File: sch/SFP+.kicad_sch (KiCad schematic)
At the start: 13 parts, among them J14 Conn_01x02_Pin, J15 Conn_01x02_Pin, J16 TE 2007262-1, J6 SFP+, J7 SFP+

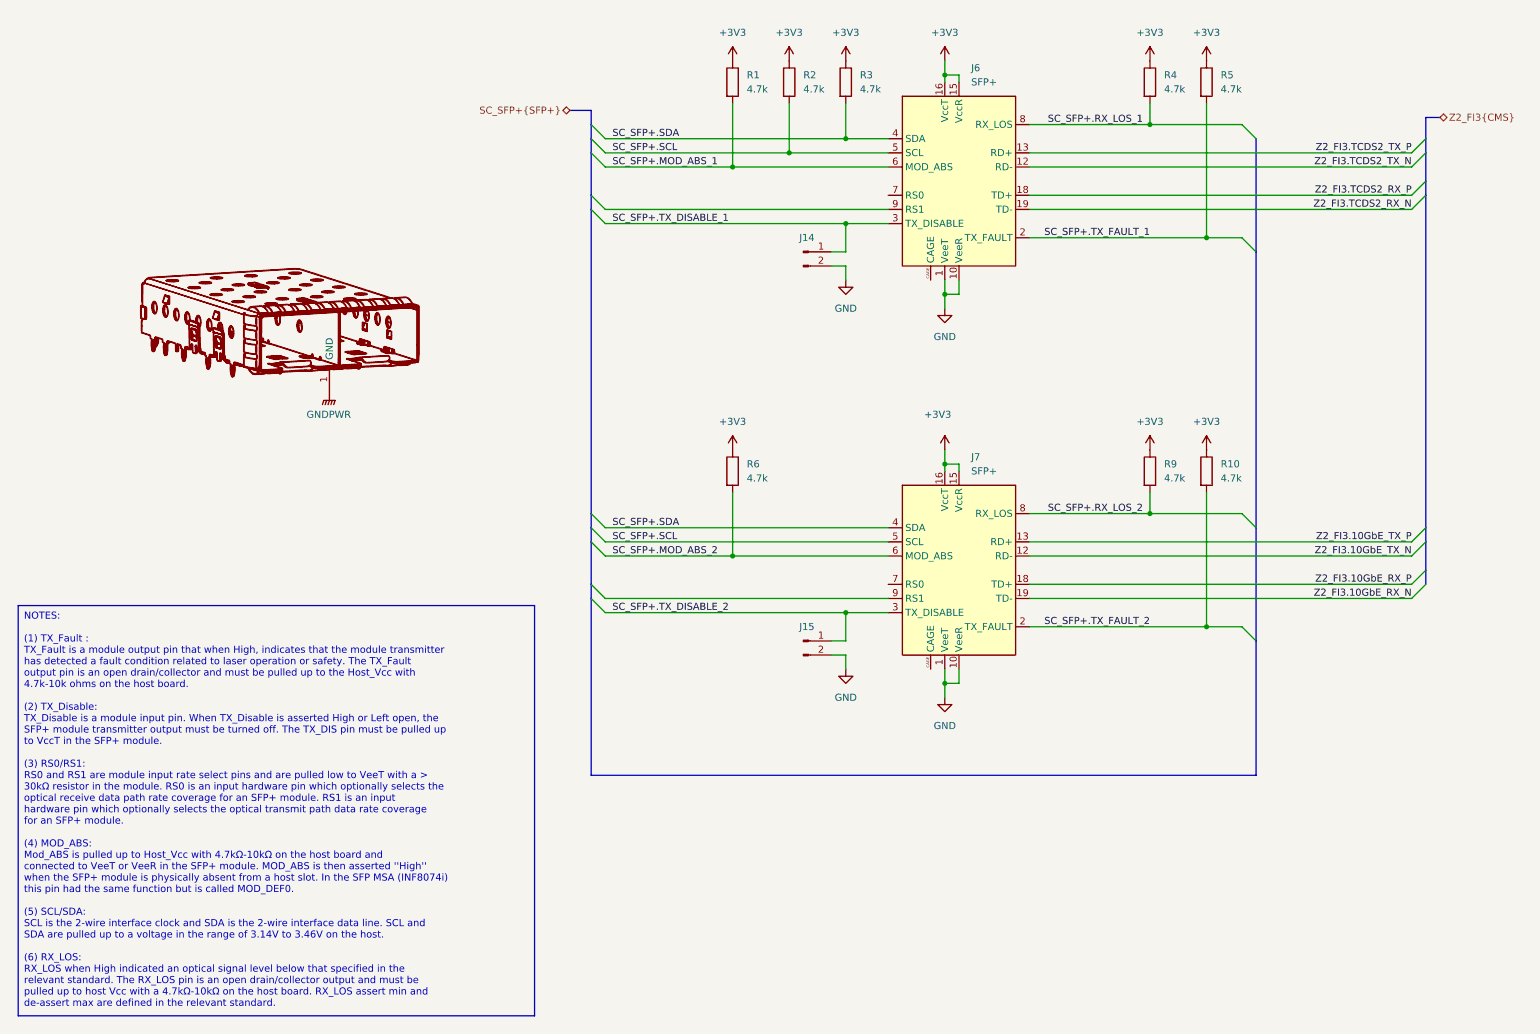
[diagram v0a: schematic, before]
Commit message: sch work
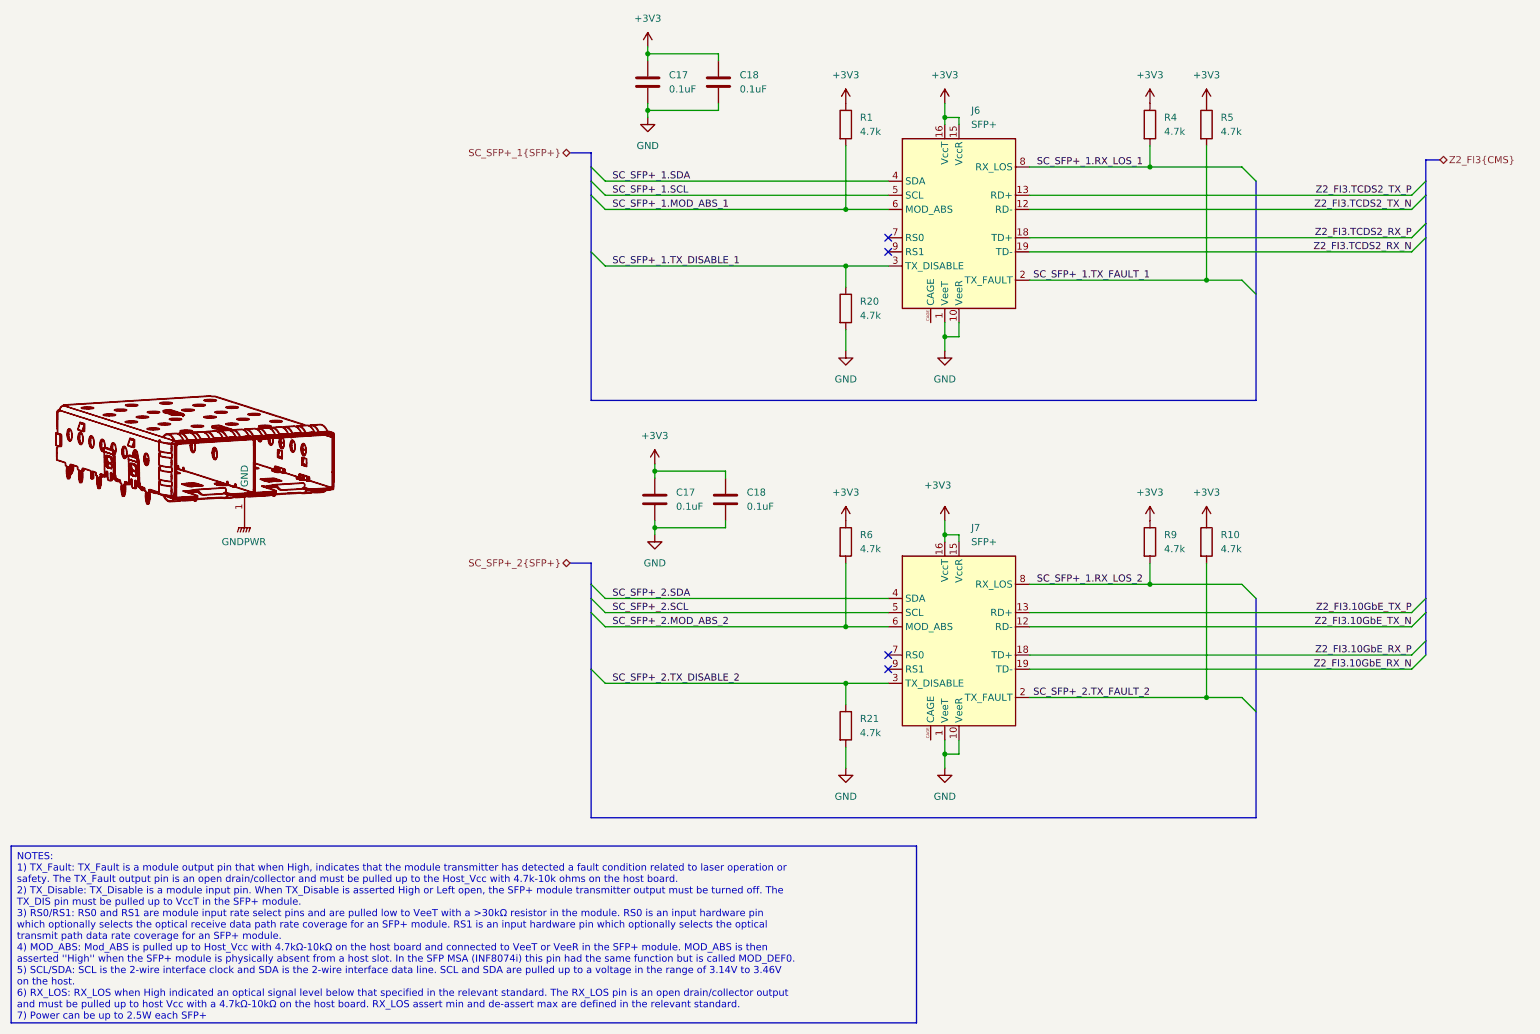
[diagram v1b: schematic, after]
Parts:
- removed J14, J15: Conn_01x02_Pin, Connector_PinHeader_2.54mm:PinHeader_1x02_P2.54mm_Vertical, symbol Connector:Conn_01x02_Pin
- removed R2, R3: 4.7k, Resistor_SMD:R_0402_1005Metric, symbol Device:R
- added C17 (x2), C18 (x2): 0.1uF, Capacitor_SMD:C_0402_1005Metric, symbol Device:C
- added R20, R21: 4.7k, Resistor_SMD:R_0402_1005Metric, symbol Device:R
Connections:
- net +3V3: now also C17.2, C17.2, C18.2, C18.2
- net GND: now also C17.1, C17.1, C18.1, C18.1, R20.2, R21.2
- net SC_SFP+.MOD_ABS_1 renamed SC_SFP+_1.MOD_ABS_1
- net SC_SFP+.MOD_ABS_2 renamed SC_SFP+_2.MOD_ABS_2
- net SC_SFP+.RX_LOS_1 renamed SC_SFP+_1.RX_LOS_1
- net SC_SFP+.RX_LOS_2 renamed SC_SFP+_1.RX_LOS_2
- net SC_SFP+.SCL renamed SC_SFP+_1.SCL
- net SC_SFP+_1.SCL: no longer J7.5 (SCL)
- net SC_SFP+.SDA renamed SC_SFP+_1.SDA
- net SC_SFP+_1.SDA: no longer J7.4 (SDA)
- net SC_SFP+.TX_DISABLE_1 renamed SC_SFP+_1.TX_DISABLE_1
- net SC_SFP+_1.TX_DISABLE_1: now also R20.1
- net SC_SFP+.TX_DISABLE_2 renamed SC_SFP+_2.TX_DISABLE_2
- net SC_SFP+_2.TX_DISABLE_2: now also R21.1
- net SC_SFP+.TX_FAULT_1 renamed SC_SFP+_1.TX_FAULT_1
- net SC_SFP+.TX_FAULT_2 renamed SC_SFP+_2.TX_FAULT_2
- new net SC_SFP+_2.SCL: J7.5 (SCL)
- new net SC_SFP+_2.SDA: J7.4 (SDA)
- no-connect marks 0 -> 4
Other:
- moved on the sheet: J6, J7, R1, R10, R4, R5, R6, R9
